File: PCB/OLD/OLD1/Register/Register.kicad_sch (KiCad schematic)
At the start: 120 parts, among them J1 Conn_01x24, J2 Conn_01x24, J3 Conn_01x24, U1 74HCT574, U13 74LS21, U14 74LS21, U15 74LS21, U16 74LS21, U2 74HCT574, U3 74LS541, U4 74LS541, U5 74HCT574, U6 74LS541

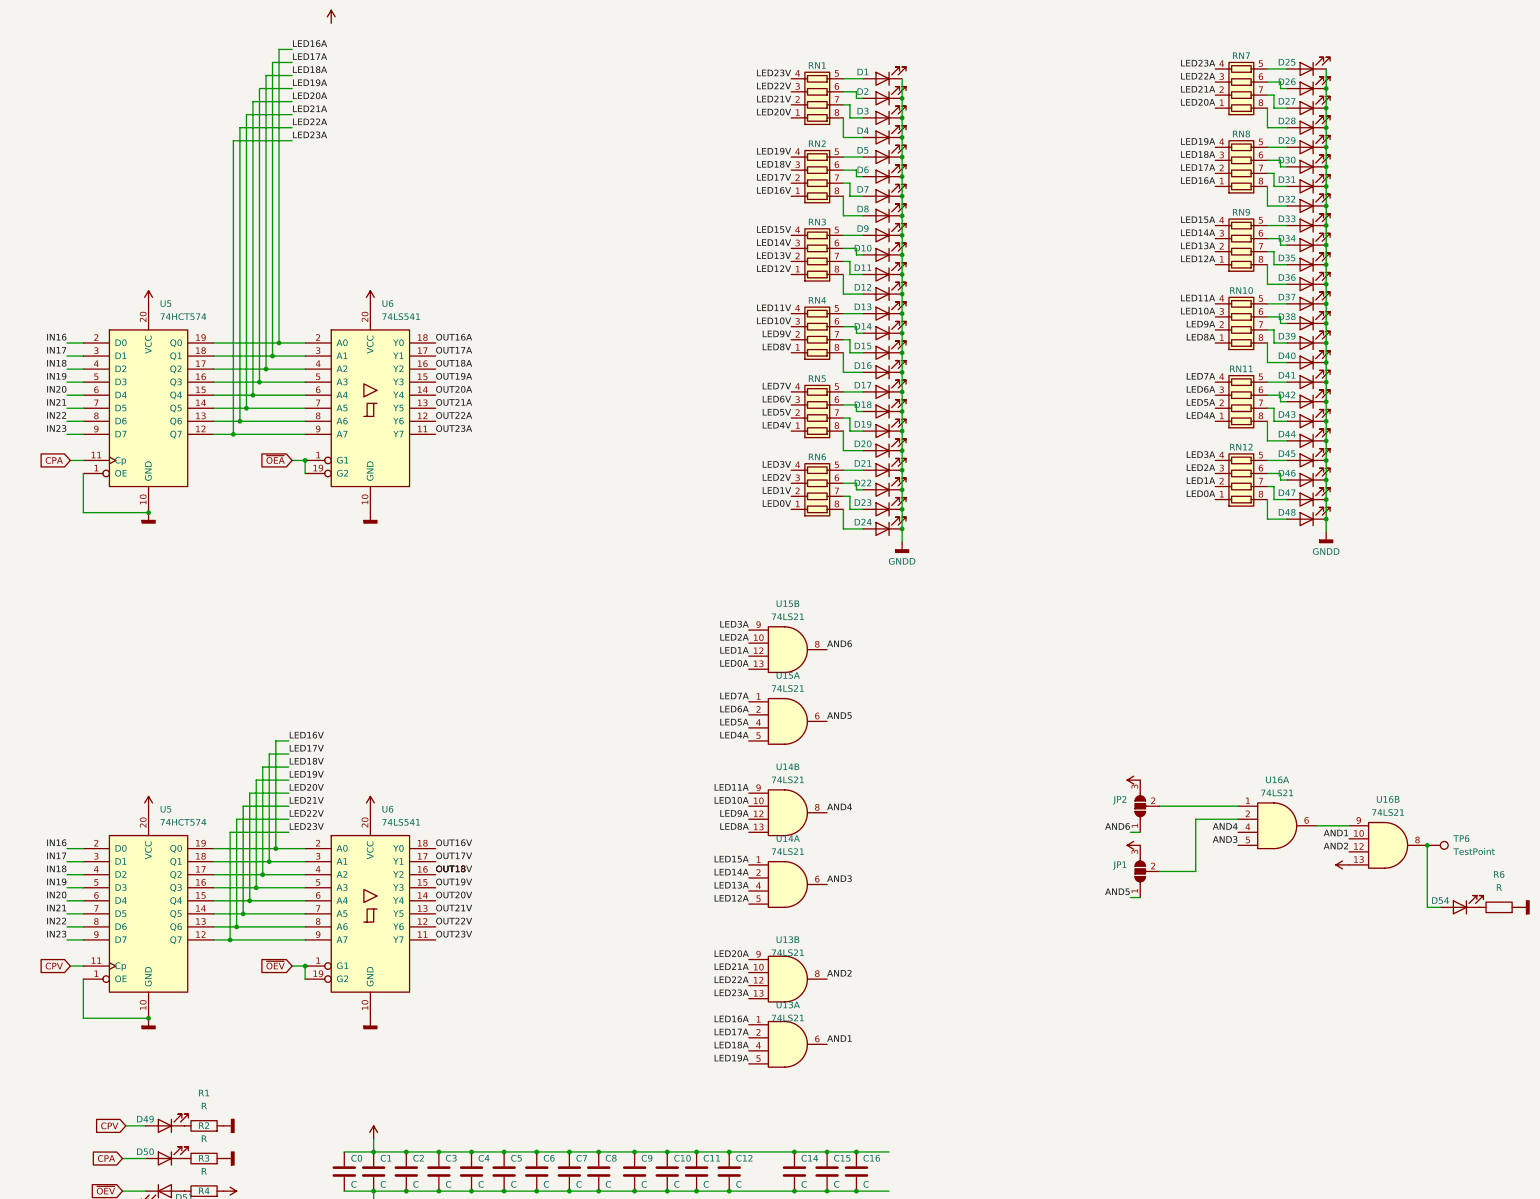
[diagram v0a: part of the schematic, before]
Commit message: WIP
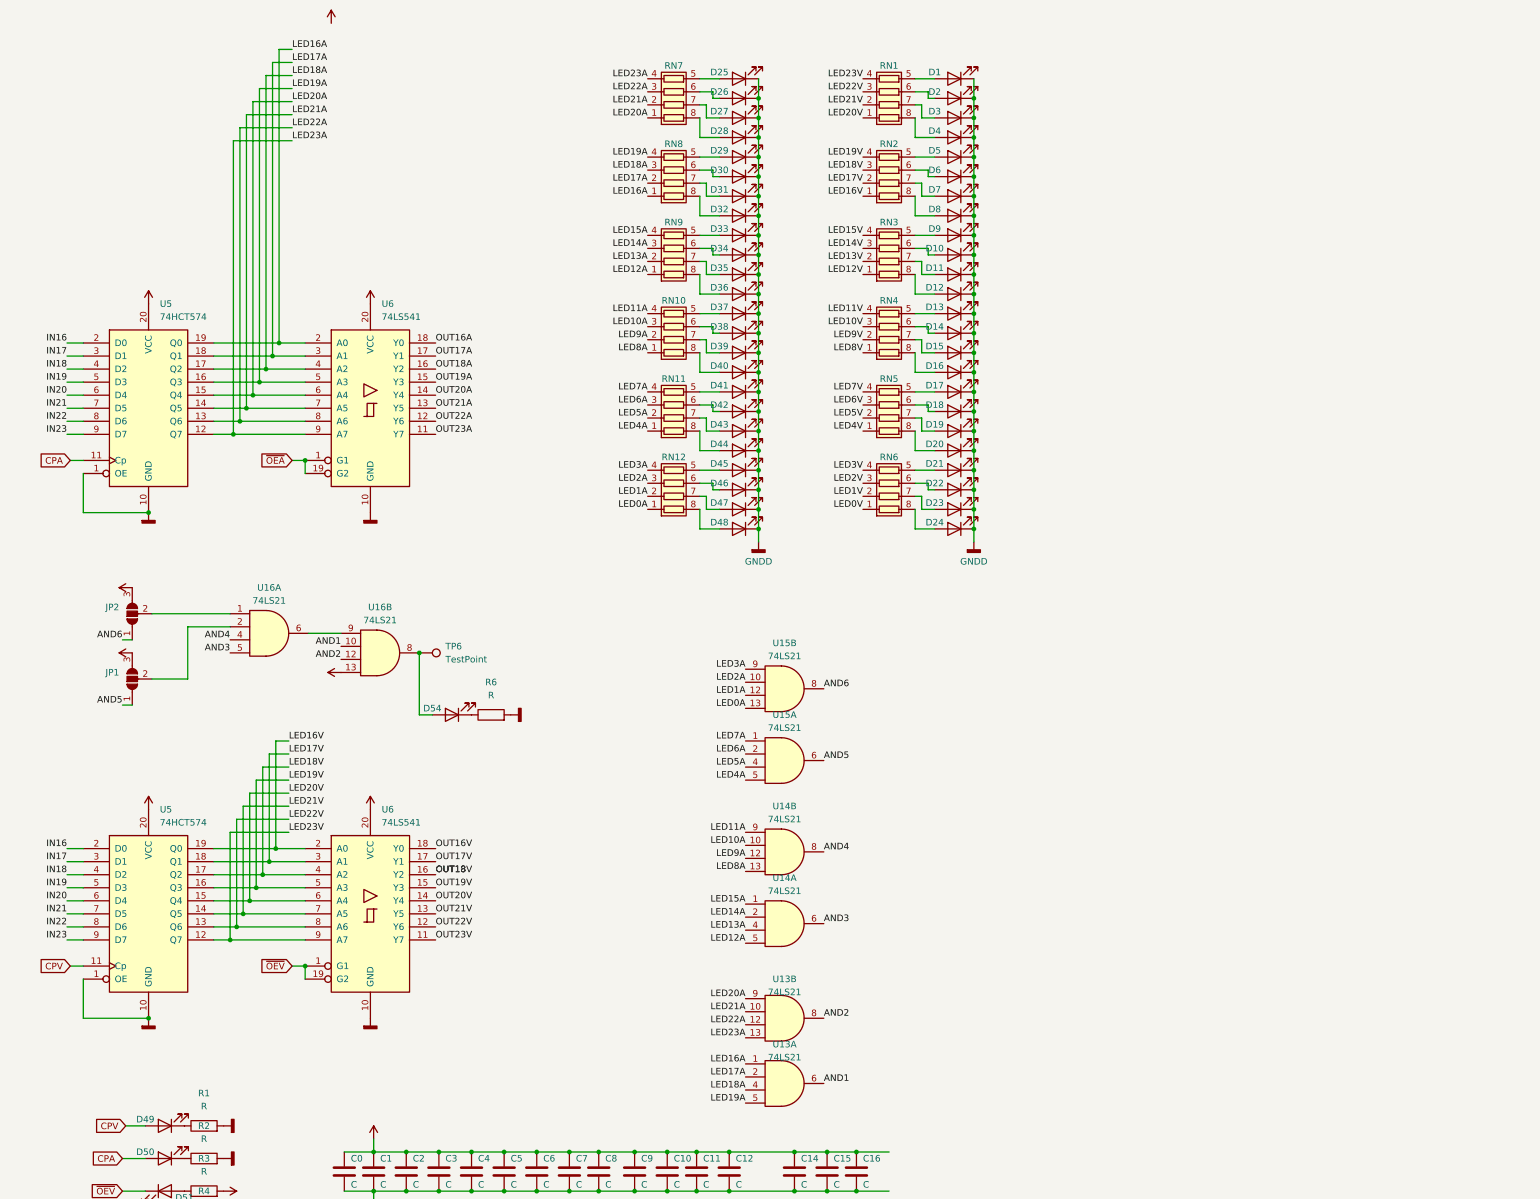
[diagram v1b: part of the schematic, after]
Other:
- moved on the sheet: D1, D10, D11, D12, D13, D14, D15, D16, D17, D18, D19, D2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
